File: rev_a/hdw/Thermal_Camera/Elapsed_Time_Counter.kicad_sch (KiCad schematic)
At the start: 10 parts, among them U502 MCP9804

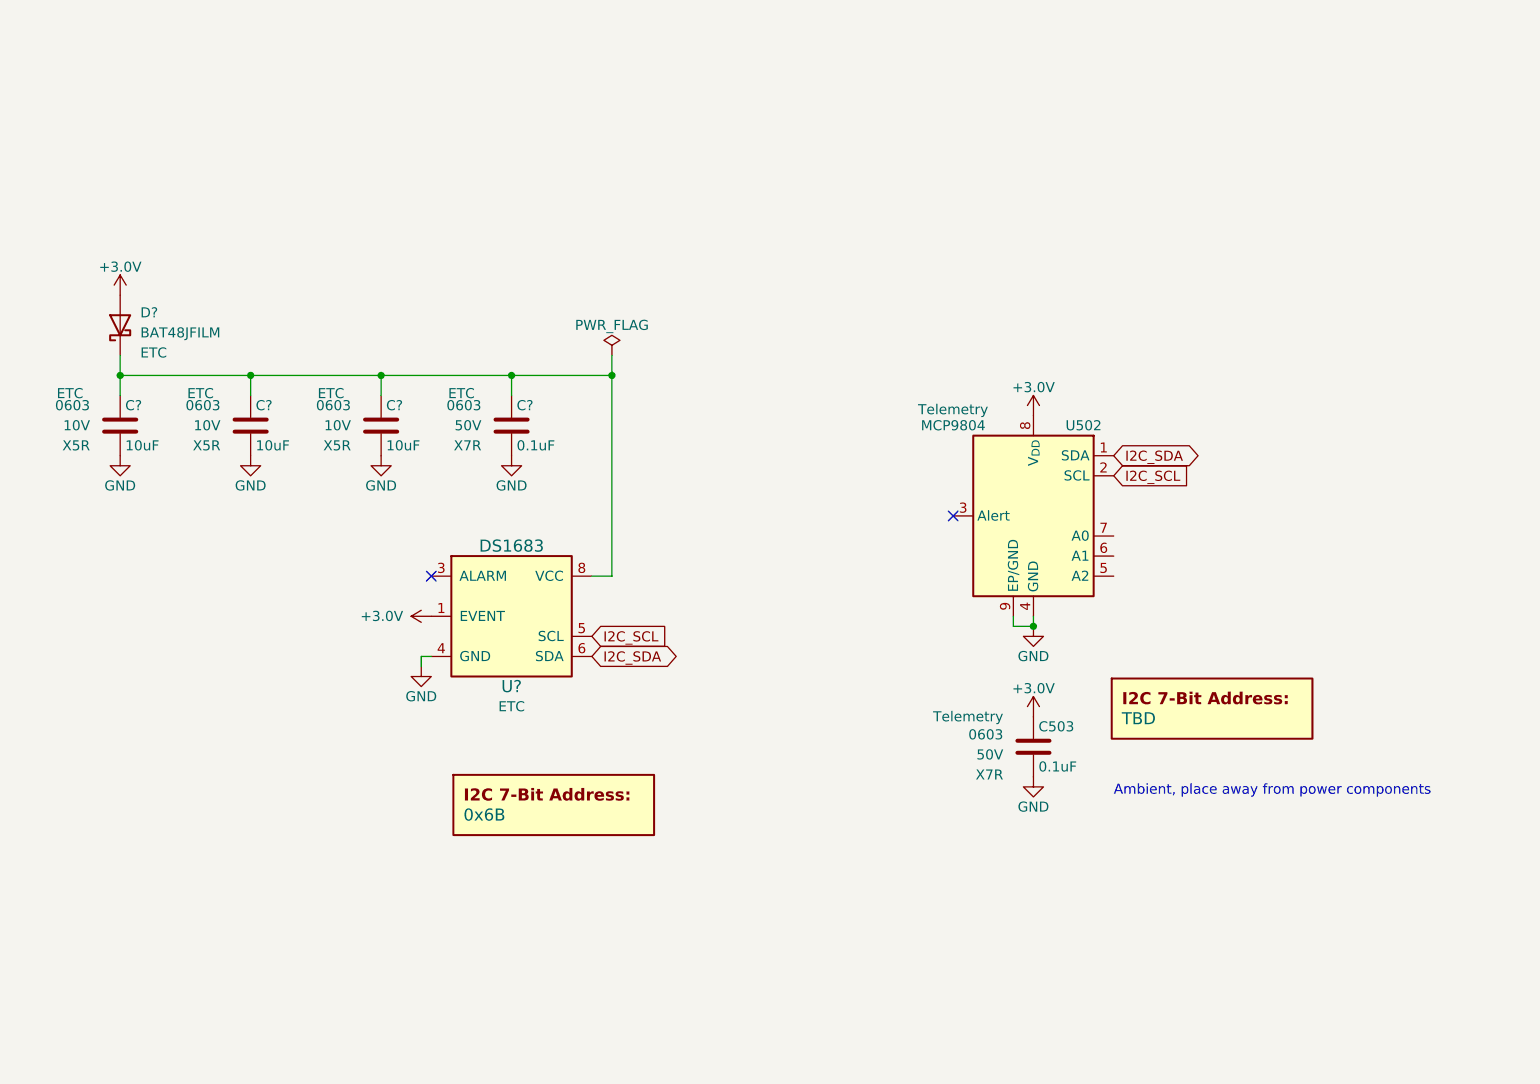
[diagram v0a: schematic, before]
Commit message: lots of random schematic progress
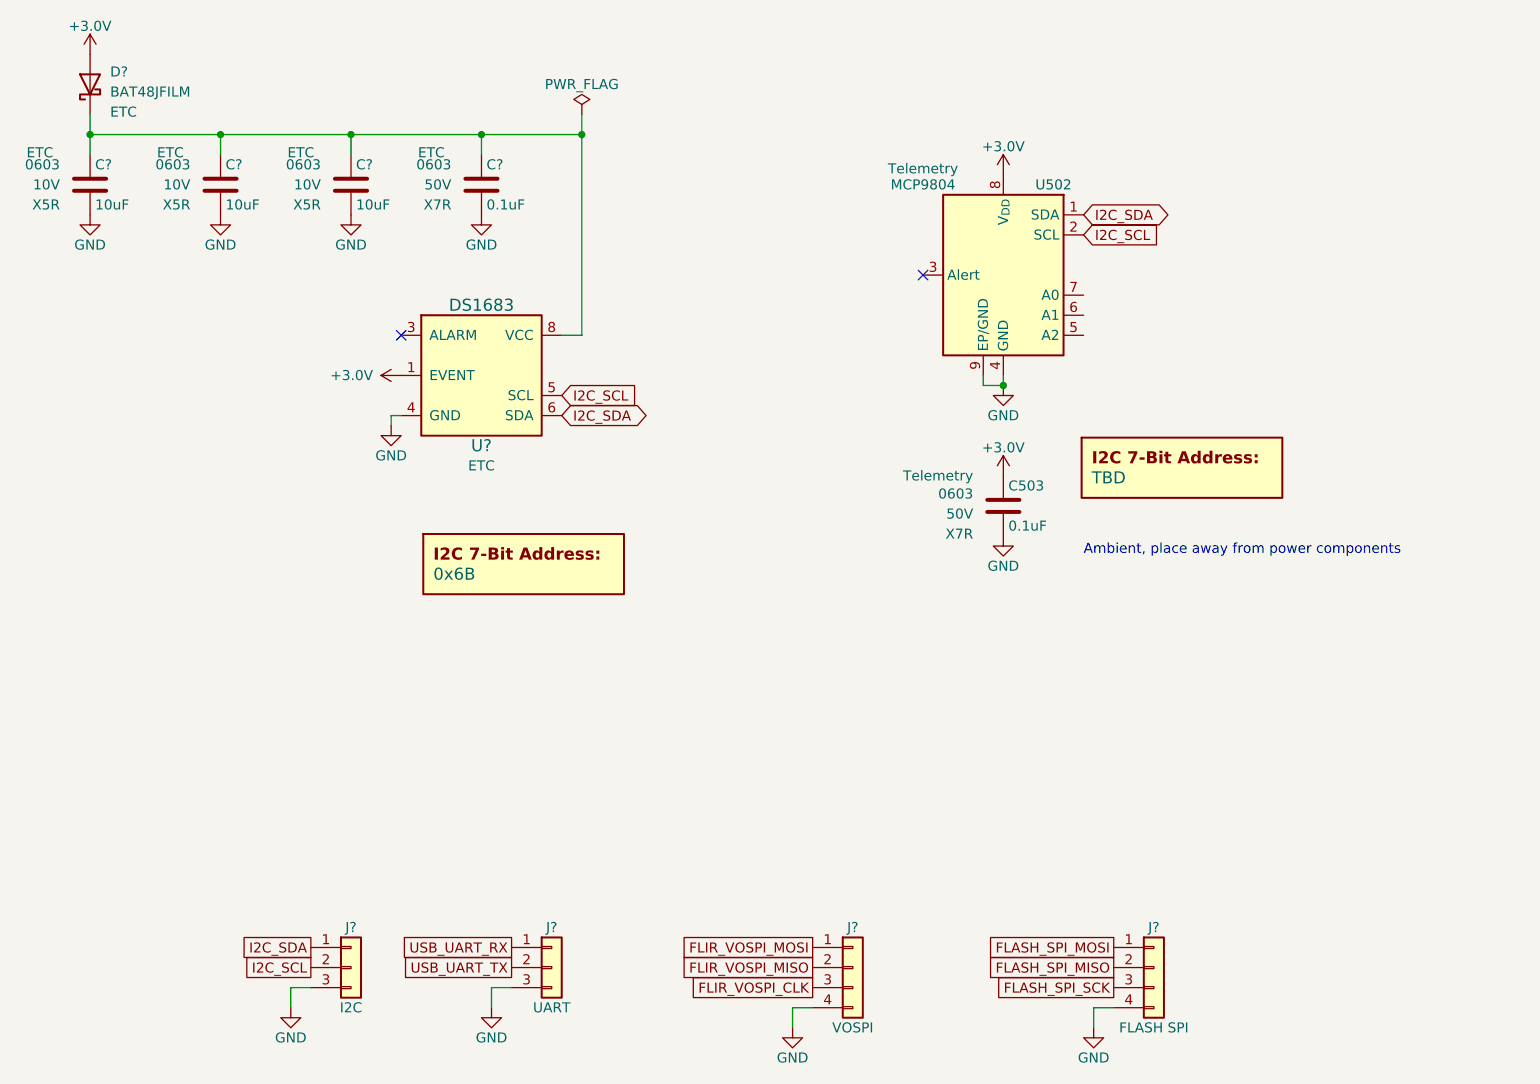
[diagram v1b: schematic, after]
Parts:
- added J?: VOSPI, symbol Connector_Generic:Conn_01x04
- added J?: FLASH SPI, symbol Connector_Generic:Conn_01x04
- added J?: I2C, symbol Connector_Generic:Conn_01x03
- added J?: UART, symbol Connector_Generic:Conn_01x03
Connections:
- net GND: now also J?.3 (Pin_3), J?.3 (Pin_3), J?.4 (Pin_4), J?.4 (Pin_4)
- net I2C_SCL: now also J?.2 (Pin_2)
- net I2C_SDA: now also J?.1 (Pin_1)
- new net FLASH_SPI_MISO: J?.2 (Pin_2)
- new net FLASH_SPI_MOSI: J?.1 (Pin_1)
- new net FLASH_SPI_SCK: J?.3 (Pin_3)
- new net FLIR_VOSPI_CLK: J?.3 (Pin_3)
- new net FLIR_VOSPI_MISO: J?.2 (Pin_2)
- new net FLIR_VOSPI_MOSI: J?.1 (Pin_1)
- new net USB_UART_RX: J?.1 (Pin_1)
- new net USB_UART_TX: J?.2 (Pin_2)
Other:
- moved on the sheet: C503, C?, D?, U502, U?
